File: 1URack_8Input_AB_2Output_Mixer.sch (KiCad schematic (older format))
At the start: 57 parts

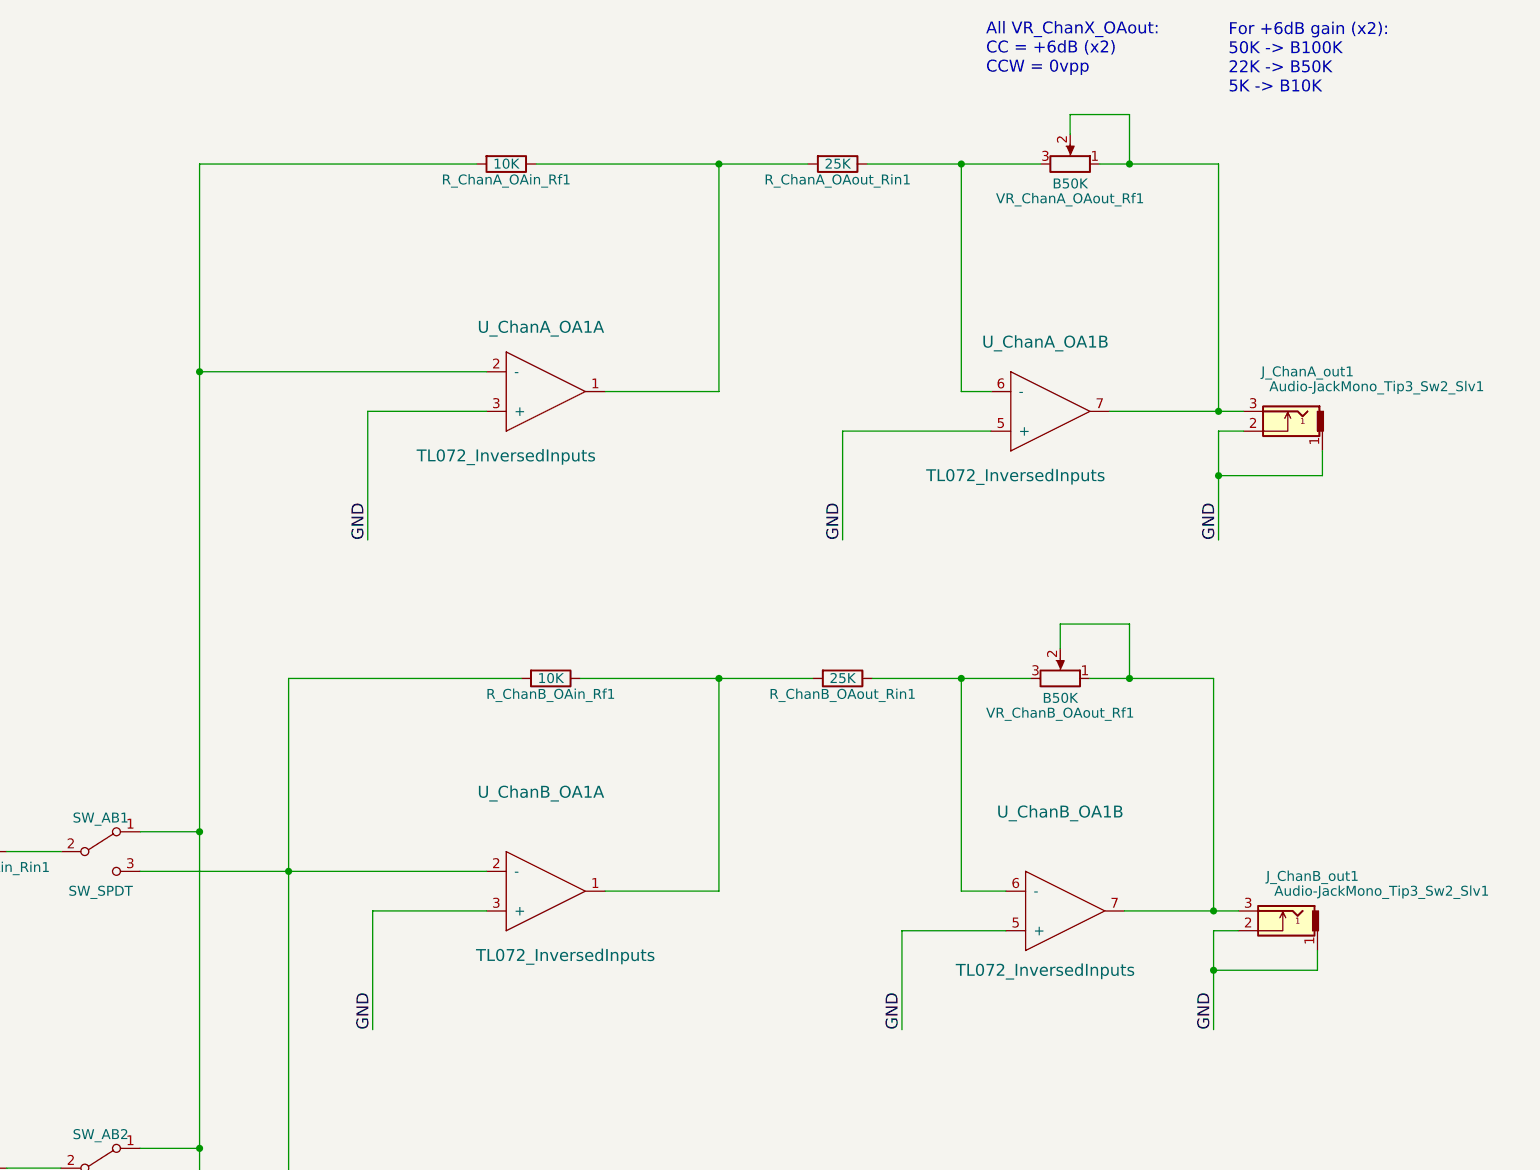
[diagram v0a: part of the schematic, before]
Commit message: First draft board layout
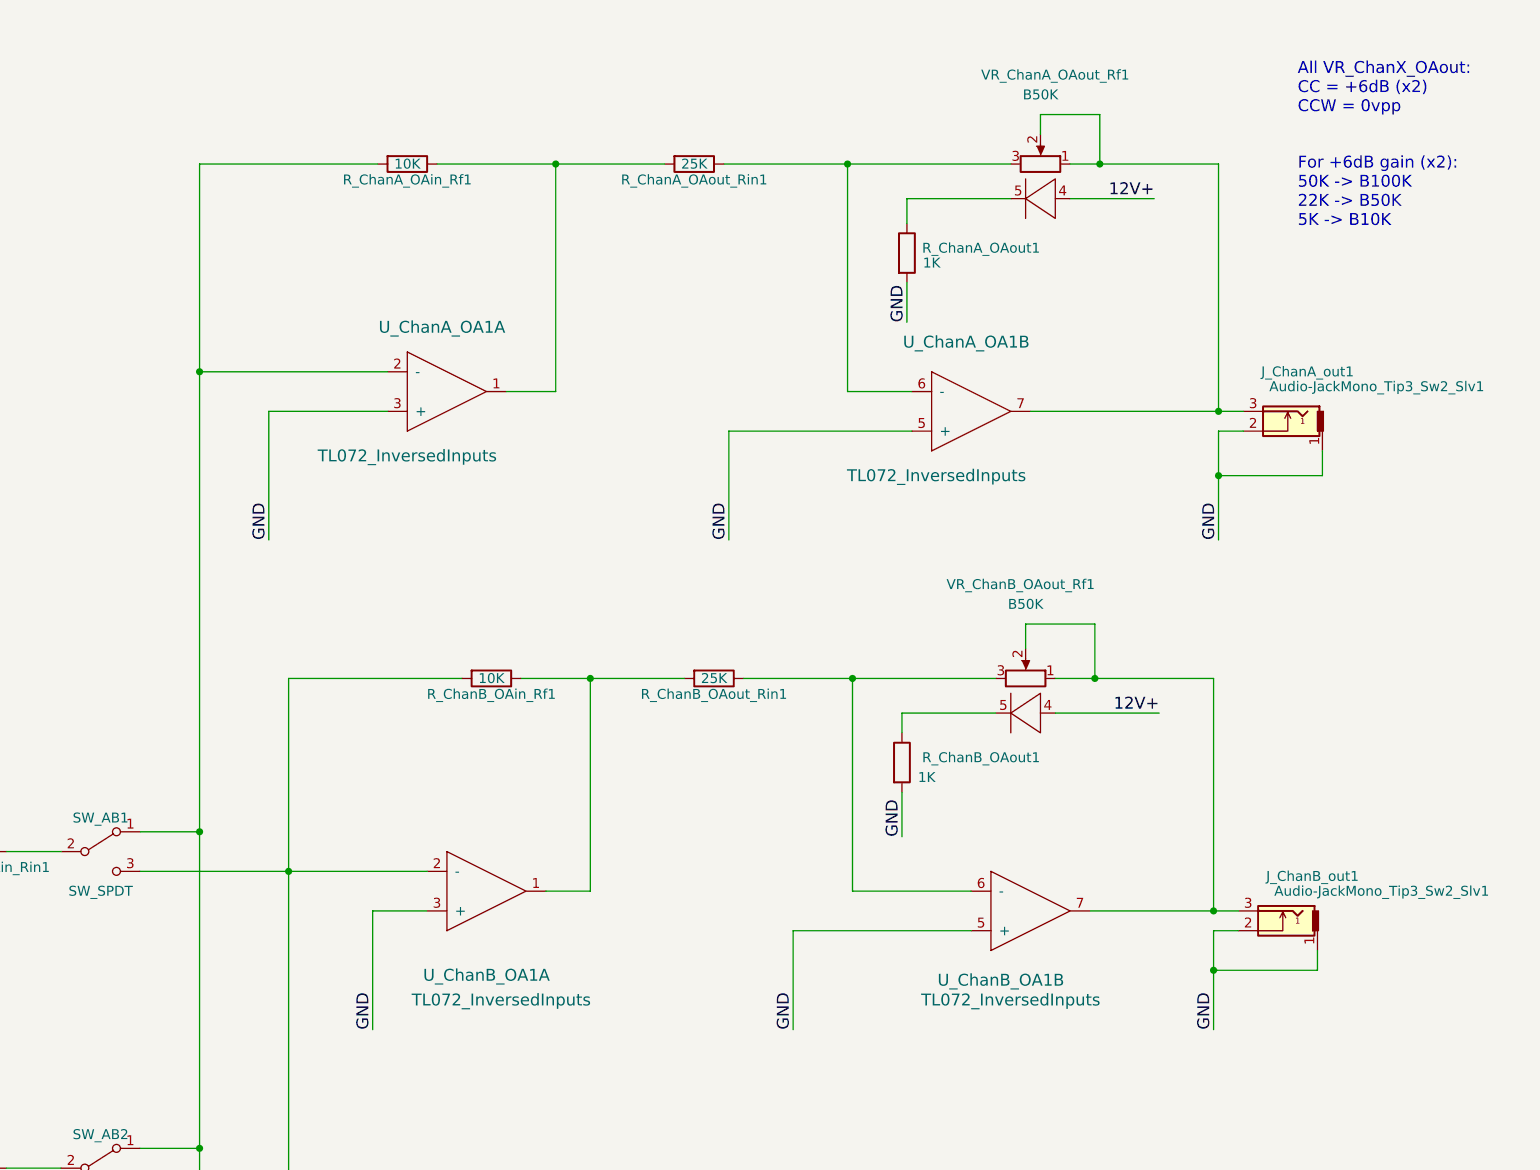
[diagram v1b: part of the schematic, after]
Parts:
- removed VR_ChanA_OAout_Rf1, VR_ChanB_OAout_Rf1: B50K, Bourn_PTL_Slider:Slider_PTL20_LED_35MM, symbol NPOT
- added R_ChanA_OAout1, R_ChanB_OAout1: 1K, Resistors_SMD:R_0805_HandSoldering, symbol R
- added VR_ChanA_OAout_Rf1, VR_ChanB_OAout_Rf1: B50K, Bourn_PTL_Slider:Slider_PTL20_LED_35MM, symbol NPOT_LED
- J_ChanA_out1, J_ChanB_out1, J_IN1, J_IN2, J_IN3, J_IN4, J_IN5, J_IN6, J_IN7, J_IN8: footprint ThonkiConn_3:Conn_3.5mmJackMono_Vertical_PJ301BM -> ThonkiConn_3:Conn_3.5mmJackMono_Vertical_PJ301M-12
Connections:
- net 12V+: now also VR_ChanA_OAout_Rf1.4, VR_ChanB_OAout_Rf1.4
- net GND: now also R_ChanA_OAout1.2, R_ChanB_OAout1.2
- net at R_ChanA_OAout_Rin1.1, U_ChanA_OA1.6 (-): now also VR_ChanA_OAout_Rf1.3
- net at R_ChanB_OAout_Rin1.1, U_ChanB_OA1.6 (-): now also VR_ChanB_OAout_Rf1.3
- net at J_ChanA_out1.3, U_ChanA_OA1.7: now also VR_ChanA_OAout_Rf1.1, VR_ChanA_OAout_Rf1.2
- net at J_ChanB_out1.3, U_ChanB_OA1.7: now also VR_ChanB_OAout_Rf1.1, VR_ChanB_OAout_Rf1.2
- new net: R_ChanA_OAout1.1, VR_ChanA_OAout_Rf1.5
- new net: R_ChanB_OAout1.1, VR_ChanB_OAout_Rf1.5
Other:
- moved on the sheet: R_ChanA_OAin_Rf1, R_ChanA_OAout_Rin1, R_ChanB_OAin_Rf1, R_ChanB_OAout_Rin1, U_ChanA_OA1A, U_ChanA_OA1B, U_ChanB_OA1A, U_ChanB_OA1B
